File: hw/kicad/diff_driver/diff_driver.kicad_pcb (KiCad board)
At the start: 2 copper layers, 32 x 22 mm, 11 parts, among them J1 CONN_01X05, J2 RJ45_LED, U1 LTC1688

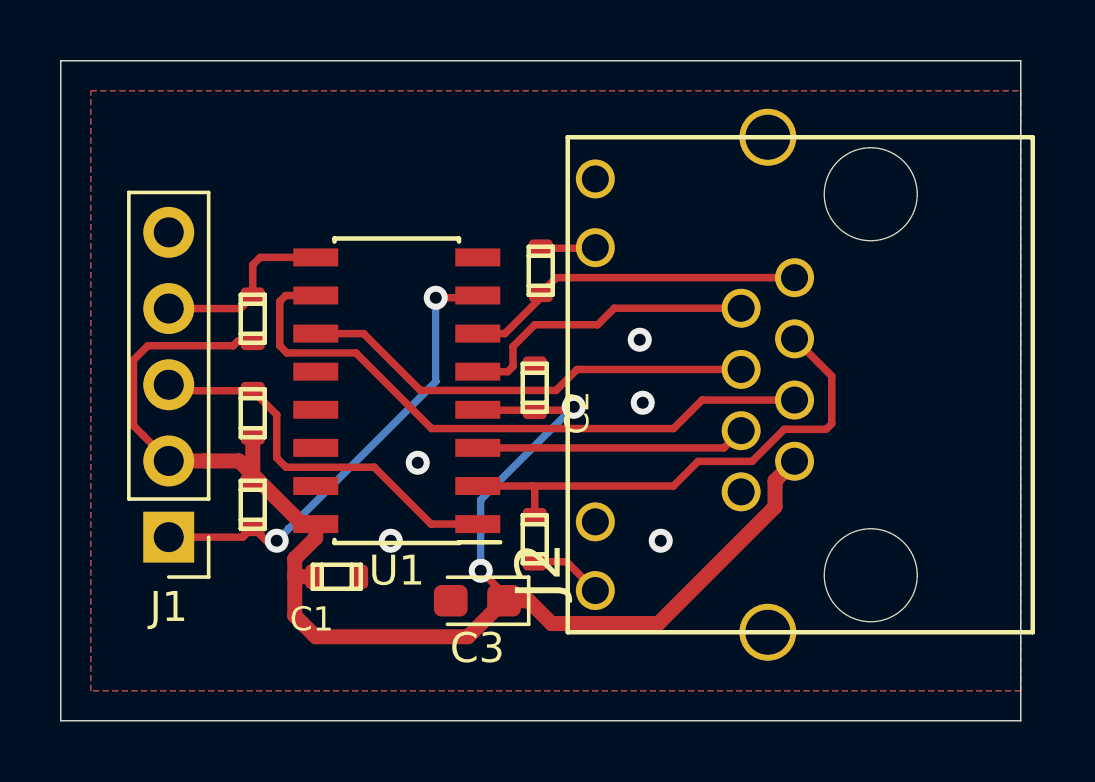
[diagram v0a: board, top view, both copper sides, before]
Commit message: flip layout
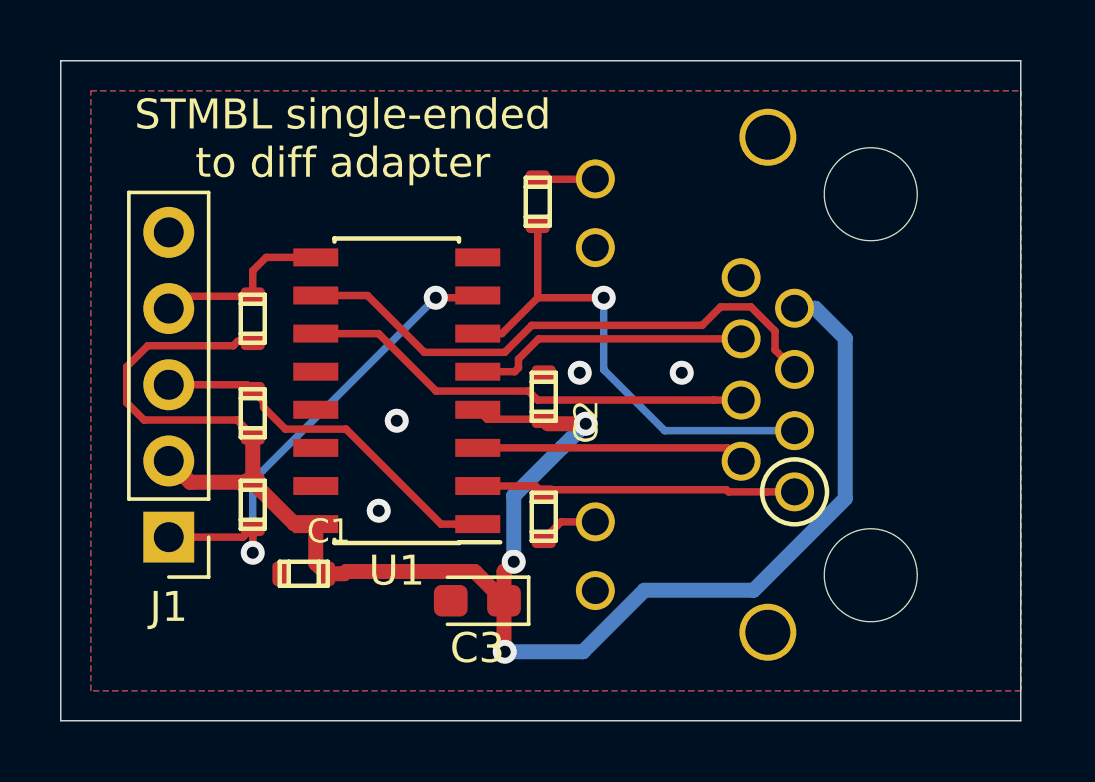
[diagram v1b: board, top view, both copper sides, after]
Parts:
- J2: moved to B.Cu
- moved R5 11.3 mm to (158.9, 84.7), turned to 90 degrees
- moved R4 8.20 mm to (159.1, 95.2), turned to 270 degrees
- moved C1 1.10 mm to (151.1, 97.1), turned to 180 degrees
- moved C2 0.42 mm to (159.1, 91.2)
- turned J2 to 90 degrees
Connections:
- U1 pad 2: Net-(J2-Pad3) -> Net-(J2-Pad1)
- U1 pad 3: Net-(J2-Pad6) -> Net-(J2-Pad2)
- U1 pad 5: Net-(J2-Pad2) -> Net-(J2-Pad6)
- U1 pad 6: Net-(J2-Pad1) -> Net-(J2-Pad3)
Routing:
- net +5V: track 51.2 -> 59.4 mm, vias 2 -> 3
- net Net-(J2-Pad5): track 21.5 -> 18.6 mm
- net Net-(J2-Pad2): track 10.0 -> 8.96 mm
- net A: track 13.1 -> 12.3 mm
- net Net-(J2-Pad1): track 11.4 -> 10.8 mm
- net B: track 15.6 -> 16.2 mm
- net Net-(J2-Pad3): track 17.1 -> 16.7 mm, vias 0 -> 1
- net GND: vias 5 -> 4
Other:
- board text added: "5V"
- board text added: "A/U"
- board text added: "B/V"
- board text added: "GND"
- board text added: "IDX/W"
- board text added: "STMBL single-ended to diff adapter"
